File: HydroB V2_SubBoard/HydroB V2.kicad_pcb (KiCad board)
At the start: 4 copper layers, 110.6 x 76.4 mm, 85 parts, among them J1 Conn_01x02_Pin, J10 Screw_Terminal_01x02, J16 Screw_Terminal_01x02, J2 Conn_01x02_Pin, J3 Screw_Terminal_01x02, J4 Conn_01x04_Pin, J5 PH SENSOR, J6 EC SENSOR, J7 Conn_01x02_Pin, J8 Screw_Terminal_01x02, J9 Screw_Terminal_01x02, Q1 S8050, Q2 S8050, Q3 S8050, Q4 S8050, Q8 S8050, SW1 SW_Push, U1 STM32F103C8Tx, U3 SN65HVD72DR, U4 LMR33620ADDA, U5 SN65HVD230, Y1 8Mhz

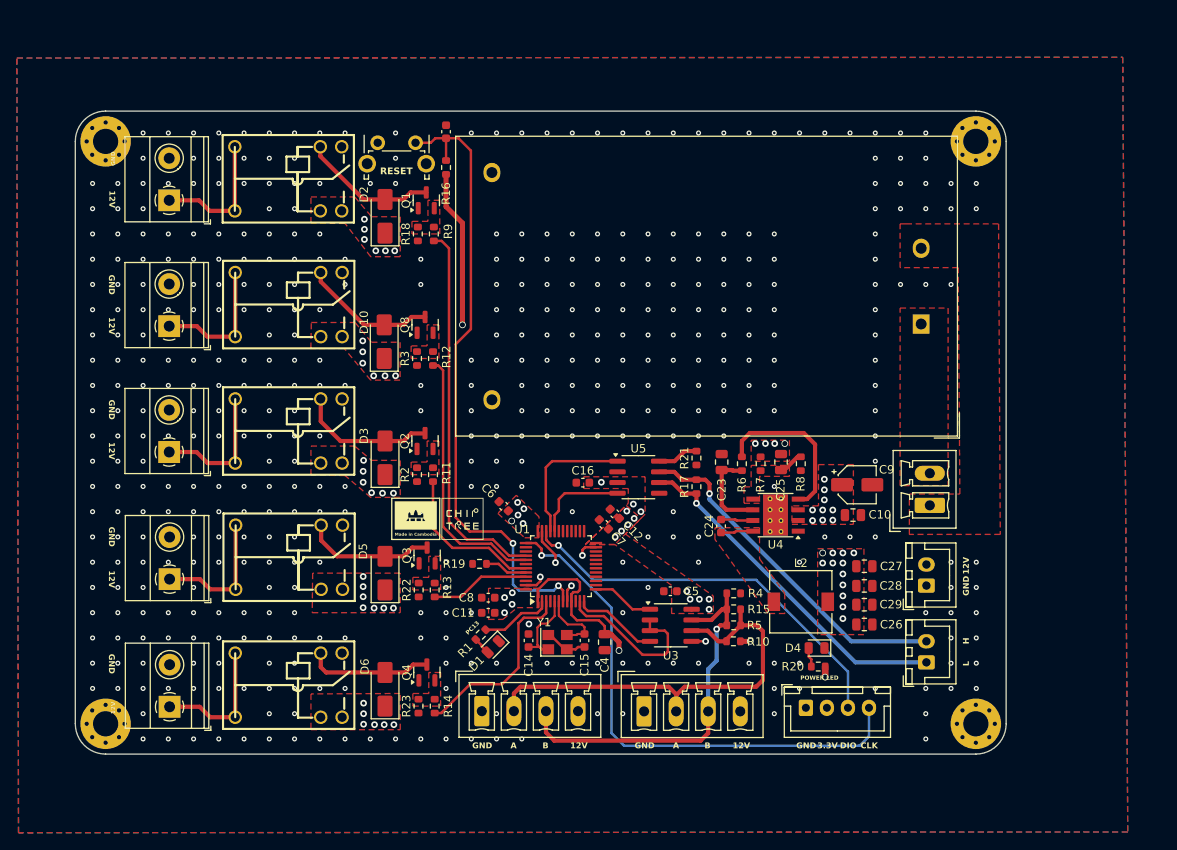
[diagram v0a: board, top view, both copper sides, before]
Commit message: subboard new update version
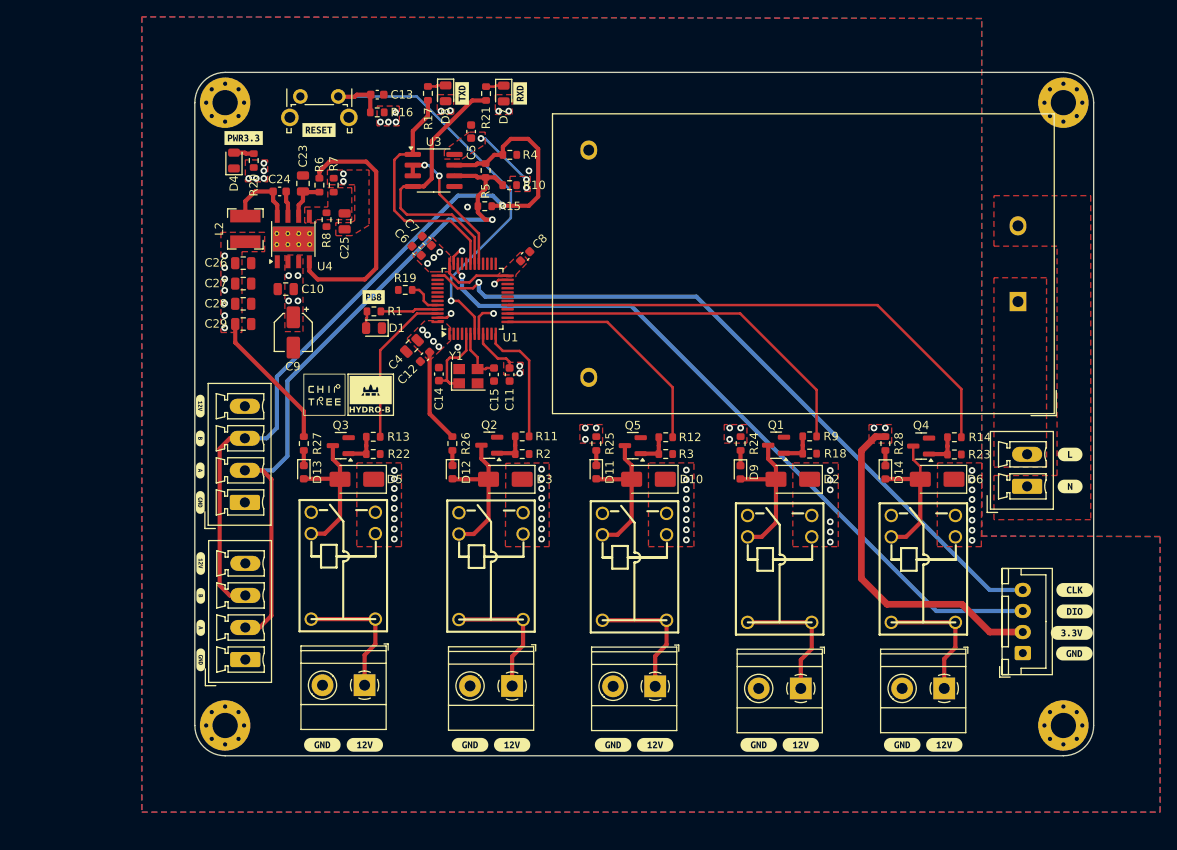
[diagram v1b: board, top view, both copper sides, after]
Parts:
- removed C16: 100nF, Capacitor_SMD:C_0603_1608Metric
- removed J1, J2: Conn_01x02_Pin, Connector_JST:JST_XH_B2B-XH-A_1x02_P2.50mm_Vertical
- removed Q8: S8050, Package_TO_SOT_SMD:SOT-23
- removed U5: SN65HVD230, Package_SO:SOIC-8_3.9x4.9mm_P1.27mm
- added D11: LED, LED_SMD:LED_0603_1608Metric, F.Cu at (144.5, 103.1)
- added D12: LED, LED_SMD:LED_0603_1608Metric, F.Cu at (127.4, 103.1)
- added D13: LED, LED_SMD:LED_0603_1608Metric, F.Cu at (109.8, 103.1)
- added D14: LED, LED_SMD:LED_0603_1608Metric, F.Cu at (178.8, 103.1)
- added D7: LED_Small, LED_SMD:LED_0805_2012Metric, F.Cu at (133.5, 58.1)
- added D8: LED_Small, LED_SMD:LED_0805_2012Metric, F.Cu at (126.6, 58.1)
- added D9: LED, LED_SMD:LED_0603_1608Metric, F.Cu at (161.6, 103.1)
- added Q5: S8050, Package_TO_SOT_SMD:SOT-23, F.Cu at (148.8, 100.0)
- added R24: 1K, Resistor_SMD:R_0603_1608Metric, F.Cu at (161.7, 99.7)
- added R25: 1K, Resistor_SMD:R_0603_1608Metric, F.Cu at (144.5, 99.7)
- added R26: 1K, Resistor_SMD:R_0603_1608Metric, F.Cu at (127.4, 99.7)
- added R27: 1K, Resistor_SMD:R_0603_1608Metric, F.Cu at (109.8, 99.7)
- added R28: 1K, Resistor_SMD:R_0603_1608Metric, F.Cu at (178.8, 99.7)
- added kibuzzard-668BA666: G***, kibuzzard-668BA666, F.Cu at (118.0, 82.3)
- added kibuzzard-668BA6B4: G***, kibuzzard-668BA6B4, F.Cu at (128.6, 58.1)
- added kibuzzard-668BA6C7: G***, kibuzzard-668BA6C7, F.Cu at (135.4, 58.1)
- added kibuzzard-668BA6F1: G***, kibuzzard-668BA6F1, F.Cu at (102.6, 63.4)
- added kibuzzard-668BA7A5: G***, kibuzzard-668BA7A5, F.Cu at (111.5, 62.5)
- added kibuzzard-668BA7C8: G***, kibuzzard-668BA7C8, F.Cu at (200.8, 104.8)
- added kibuzzard-668BA7EF: G***, kibuzzard-668BA7EF, F.Cu at (200.8, 101.0)
- added kibuzzard-668BA811: G***, kibuzzard-668BA811, F.Cu at (201.3, 117.1)
- added kibuzzard-668BA833: G***, kibuzzard-668BA833, F.Cu at (201.3, 119.7)
- added kibuzzard-668BA852: G***, kibuzzard-668BA852, F.Cu at (201.0, 122.2)
- added kibuzzard-668BA86D: G***, kibuzzard-668BA86D, F.Cu at (201.3, 124.7)
- added kibuzzard-668BA998: G***, kibuzzard-668BA998, F.Cu at (97.5, 95.2)
- added kibuzzard-668BA998: G***, kibuzzard-668BA998, F.Cu at (97.5, 114.0)
- added kibuzzard-668BA9FB: G***, kibuzzard-668BA9FB, F.Cu at (97.5, 121.6)
- added kibuzzard-668BA9FB: G***, kibuzzard-668BA9FB, F.Cu at (97.5, 102.9)
- added kibuzzard-668BAA24: G***, kibuzzard-668BAA24, F.Cu at (97.5, 117.8)
- added kibuzzard-668BAA24: G***, kibuzzard-668BAA24, F.Cu at (97.5, 99.1)
- added kibuzzard-668BAA39: G***, kibuzzard-668BAA39, F.Cu at (97.5, 106.7)
- added kibuzzard-668BAA39: G***, kibuzzard-668BAA39, F.Cu at (97.5, 125.4)
- added kibuzzard-668BAA96: G***, kibuzzard-668BAA96, F.Cu at (180.8, 135.5)
- added kibuzzard-668BAA96: G***, kibuzzard-668BAA96, F.Cu at (129.5, 135.5)
- added kibuzzard-668BAA96: G***, kibuzzard-668BAA96, F.Cu at (112.0, 135.5)
- added kibuzzard-668BAA96: G***, kibuzzard-668BAA96, F.Cu at (163.8, 135.5)
- added kibuzzard-668BAA96: G***, kibuzzard-668BAA96, F.Cu at (146.5, 135.5)
- added kibuzzard-668BAD03: G***, kibuzzard-668BAD03, F.Cu at (117.0, 135.5)
- added kibuzzard-668BAD03: G***, kibuzzard-668BAD03, F.Cu at (185.8, 135.5)
- added kibuzzard-668BAD03: G***, kibuzzard-668BAD03, F.Cu at (134.5, 135.5)
- added kibuzzard-668BAD03: G***, kibuzzard-668BAD03, F.Cu at (168.8, 135.5)
- added kibuzzard-668BAD03: G***, kibuzzard-668BAD03, F.Cu at (151.5, 135.5)
- L2: footprint Inductor_SMD:L_7.3x7.3_H3.5 -> Inductor_SMD:L_Bourns-SRN4018
- R17: value 120 -> 10k
- moved H8 115.8 mm to (100.4, 59.2)
- moved H5 113.9 mm to (200.0, 59.2)
- moved H6 113.8 mm to (200.0, 133.2)
- moved H7 113.0 mm to (100.4, 133.2)
- moved J3 94.8 mm to (168.8, 128.8), turned to 180 degrees
- moved J10 92.1 mm to (185.8, 128.8), turned to 180 degrees
- moved D4 90.3 mm to (101.5, 66.1), turned to 90 degrees
- moved R20 90.1 mm to (103.8, 66.1), turned to 90 degrees
- moved C26 85.4 mm to (102.5, 78.3)
- moved C27 81.1 mm to (102.5, 80.7)
- moved C28 81.1 mm to (102.5, 83.1)
- moved C29 81.0 mm to (102.5, 85.5)
- moved L2 79.5 mm to (102.8, 74.2), turned to -90 degrees
- moved U10 76.7 mm to (183.4, 114.6), turned to 90 degrees
- moved U7 74.6 mm to (166.3, 114.6), turned to 90 degrees
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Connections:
- Q1 pad 1: GND -> Net-(Q1-B)
- Q1 pad 2: Net-(Q1-B) -> GND
- Q2 pad 1: GND -> Net-(Q2-B)
- Q2 pad 2: Net-(Q2-B) -> GND
- Q3 pad 1: GND -> Net-(Q3-B)
- Q3 pad 2: Net-(Q3-B) -> GND
- Q4 pad 1: GND -> Net-(Q4-B)
- Q4 pad 2: Net-(Q4-B) -> GND
- R17 pad 1: Net-(J1-Pin_1) -> /HydroB/Block Sensor1/RS485_TX
- R21 pad 1: GND -> /HydroB/Block Sensor1/RS485_RX
- U1 pad 11: /HydroB/Block Sensor1/EN_RS485 -> unconnected-(U1-PA1-Pad11)
- U1 pad 12: /HydroB/Block Sensor1/RS485_RX -> /HydroB/Block Relay1/RELAY_3
- U1 pad 13: /HydroB/Block Sensor1/RS485_TX -> /HydroB/Block Relay1/RELAY_2
- U1 pad 15: unconnected-(U1-PA5-Pad15) -> /HydroB/Block Relay1/RELAY_1
- U1 pad 17: unconnected-(U1-PA7-Pad17) -> /HydroB/Block Relay1/RELAY_5
- U1 pad 2: LED -> unconnected-(U1-PC13-Pad2)
- U1 pad 29: unconnected-(U1-PA8-Pad29) -> /HydroB/Block Sensor1/EN_RS485
- U1 pad 3: /HydroB/Block Relay1/RELAY_5 -> unconnected-(U1-PC14-Pad3)
- U1 pad 30: unconnected-(U1-PA9-Pad30) -> /HydroB/Block Sensor1/RS485_RX
- U1 pad 31: unconnected-(U1-PA10-Pad31) -> /HydroB/Block Sensor1/RS485_TX
- U1 pad 32: /HydroB/Canbus tranceiver /CAN_RX -> unconnected-(U1-PA11-Pad32)
- U1 pad 33: /HydroB/Canbus tranceiver /CAN_TX -> unconnected-(U1-PA12-Pad33)
- U1 pad 40: /HydroB/Block Relay1/RELAY_1 -> unconnected-(U1-PB4-Pad40)
- U1 pad 41: /HydroB/Block Relay1/RELAY_2 -> unconnected-(U1-PB5-Pad41)
- U1 pad 43: /HydroB/Block Relay1/RELAY_3 -> unconnected-(U1-PB7-Pad43)
- U1 pad 45: /HydroB/Block Relay1/RELAY_4 -> LED
- U1 pad 46: unconnected-(U1-PB9-Pad46) -> /HydroB/Block Relay1/RELAY_4
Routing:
- net Net-(J5-Pin_3): track 45.3 -> 93.9 mm
- net Net-(J1-Pin_1): track 41.3 -> 0.00 mm, vias 1 -> 0
- net /HydroB/Block Relay1/RELAY_5: track 22.7 -> 63.8 mm
- net Net-(D8-K): track 41.2 -> 2.16 mm, vias 1 -> 0
- net SWDIO: track 47.7 -> 85.7 mm
- net Net-(J5-Pin_2): track 55.0 -> 83.3 mm, vias 0 -> 1
- net /HydroB/Block Sensor1/RS485_RX: track 10.2 -> 32.7 mm
- net NRST: track 75.4 -> 52.9 mm, vias 2 -> 1
- net SWCLK: track 63.8 -> 86.1 mm
- net /HydroB/Block Sensor1/RS485_TX: track 7.39 -> 28.9 mm
- net +3.3V: track 107.7 -> 90.6 mm
- net /HydroB/Canbus tranceiver /CAN_TX: track 16.6 -> 0.00 mm
- net /HydroB/Canbus tranceiver /CAN_RX: track 11.3 -> 0.00 mm
- net PG: track 19.5 -> 30.0 mm
- net GND: track 18.3 -> 9.69 mm, vias 454 -> 7
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- removed copper zone on F.Cu, net A
- removed copper zone on F.Cu, net Net-(Q1-B)
- removed copper zone on F.Cu, net Net-(Q2-B)
- removed copper zone on F.Cu, net Net-(Q3-B)
- removed copper zone on F.Cu, net Net-(Q4-B)
- removed copper zone on F.Cu, net Net-(Q5-B)
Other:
- board size 110.6 x 76.4 mm -> 106.8 x 81.2 mm
- board text added: "HYDRO-B"
- board text removed: "12V"
- board text removed: "3.3V"
- board text removed: "A"
- board text removed: "B"
- board text removed: "CLK"
- board text removed: "DIO"
- board text removed: "GND"
- board text removed: "H"
- board text removed: "L"
- board text removed: "Made in Cambodia"
- board text removed: "PC13"
- board text removed: "POWER LED"
- board text removed: "RESET"
